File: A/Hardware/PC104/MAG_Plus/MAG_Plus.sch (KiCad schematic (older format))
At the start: 39 parts, among them J1 RPi_GPIO, J9 Conn_01x06_Male, SW1 SW_Push, U1 Payload, U12 PIC16F1847-I_SO, U13 LP38693MP-3.3, U14 LP38693MP-3.3, U15 LP38693MP-5.0, U16 LP38693MP-3.3, U2 ISO1540

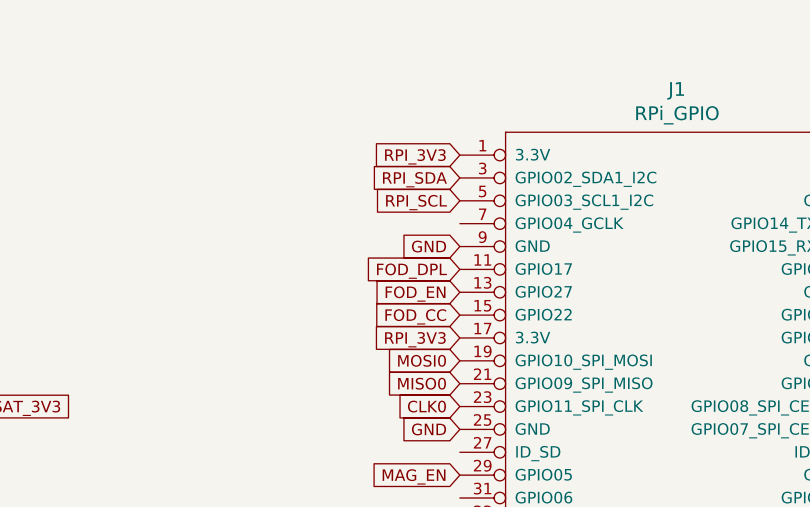
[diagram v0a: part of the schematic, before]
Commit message: Update PCBs
New version of PCBs
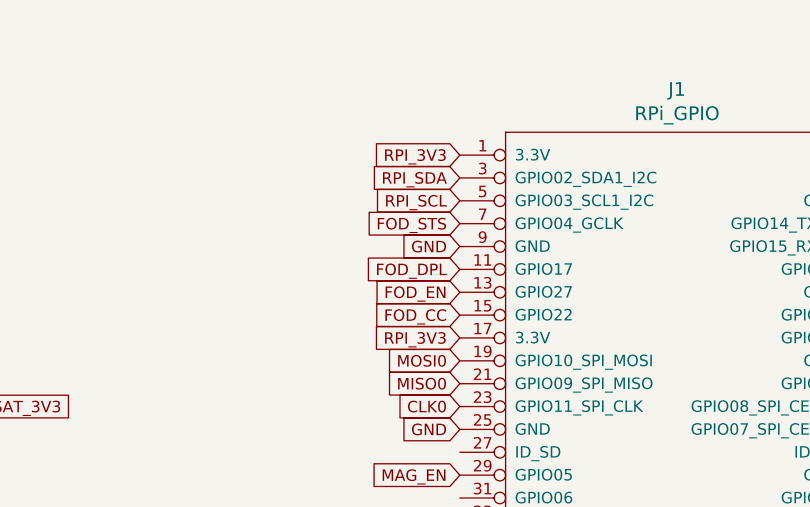
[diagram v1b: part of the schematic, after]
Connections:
- net FOD_STS: now reaches J1.7 (GPIO04_GCLK)
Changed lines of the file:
@@
 F1 "LPS.sch" 50
 $EndSheet
+Text GLabel 7600 1700 0    50   Input ~ 0
+FOD_STS
 $EndSCHEMATC

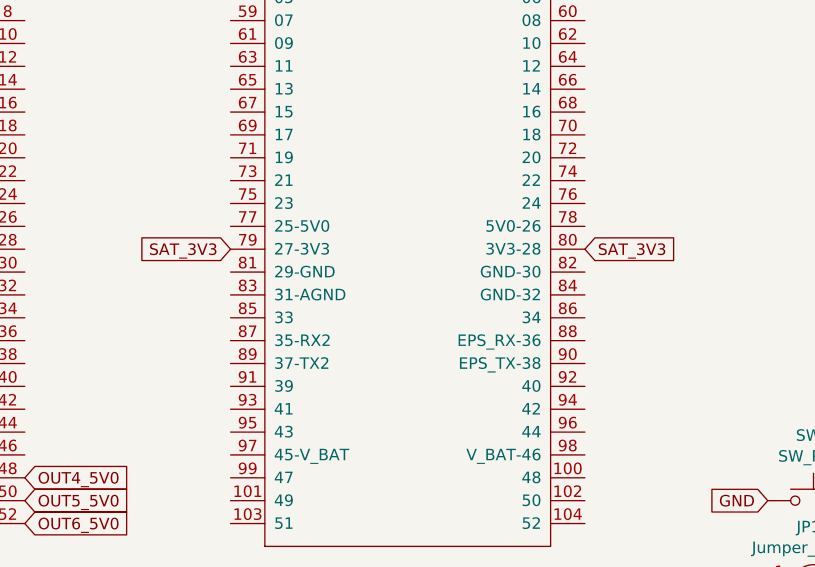
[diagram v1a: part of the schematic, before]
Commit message: minor changes
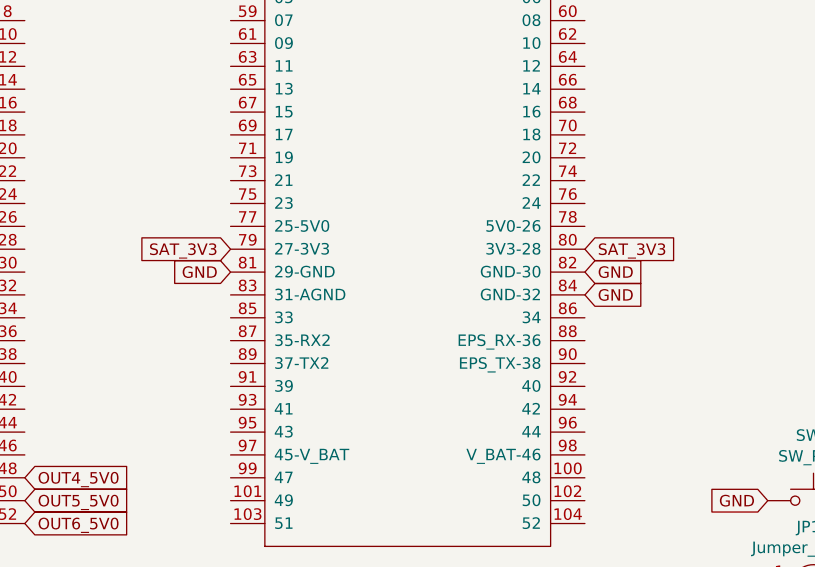
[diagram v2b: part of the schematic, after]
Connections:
- net GND: now also U1.81 (29-GND), U1.82 (GND-30), U1.84 (GND-32)
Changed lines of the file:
@@
 Text GLabel 7600 1700 0    50   Input ~ 0
 FOD_STS
+Text GLabel 3950 2600 0    50   Input ~ 0
+GND
+Text GLabel 5500 2600 2    50   Input ~ 0
+GND
+Text GLabel 5500 2700 2    50   Input ~ 0
+GND
 $EndSCHEMATC
